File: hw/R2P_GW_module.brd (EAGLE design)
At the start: 40 x 40 mm, 32 parts, among them U1 STM32F103CX, U5 LD3985XX, X1 MICROMATCH-4

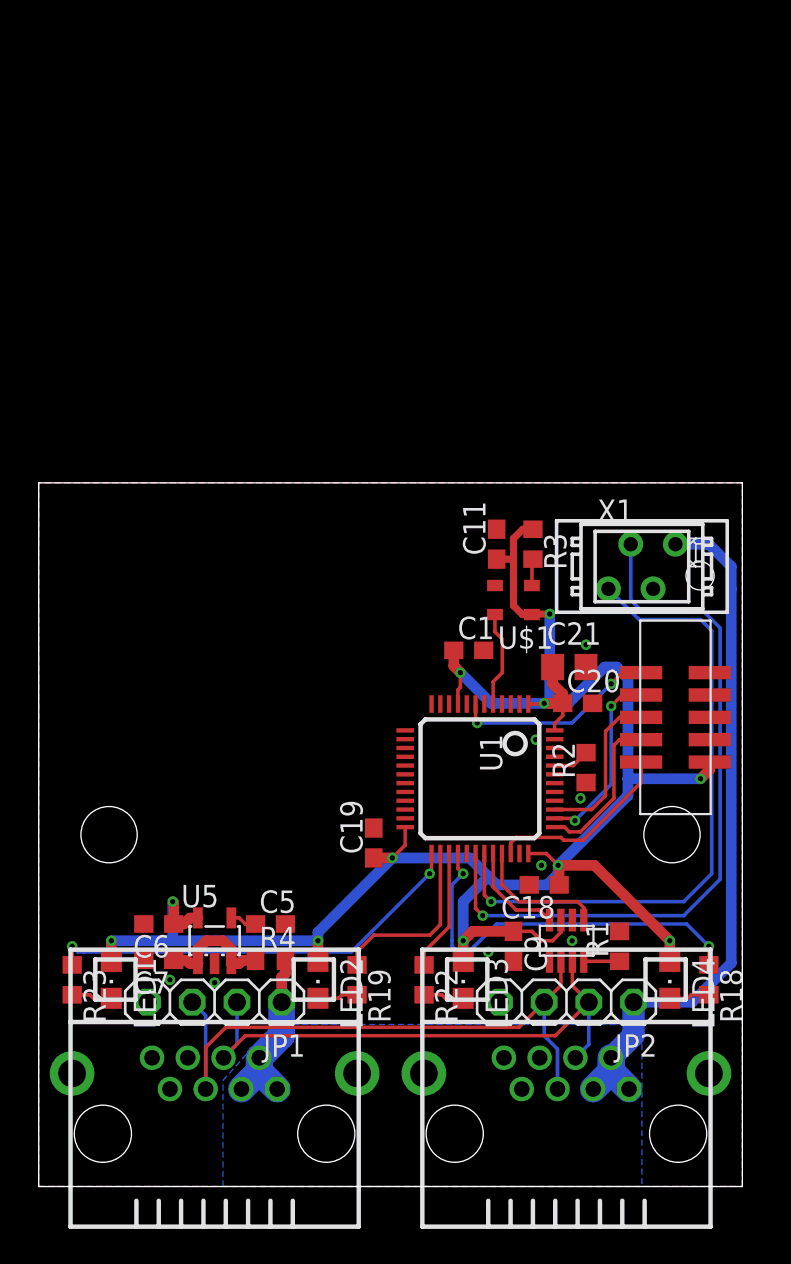
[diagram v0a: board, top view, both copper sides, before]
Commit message: First PCB version almost finished
Andrea Zoppi
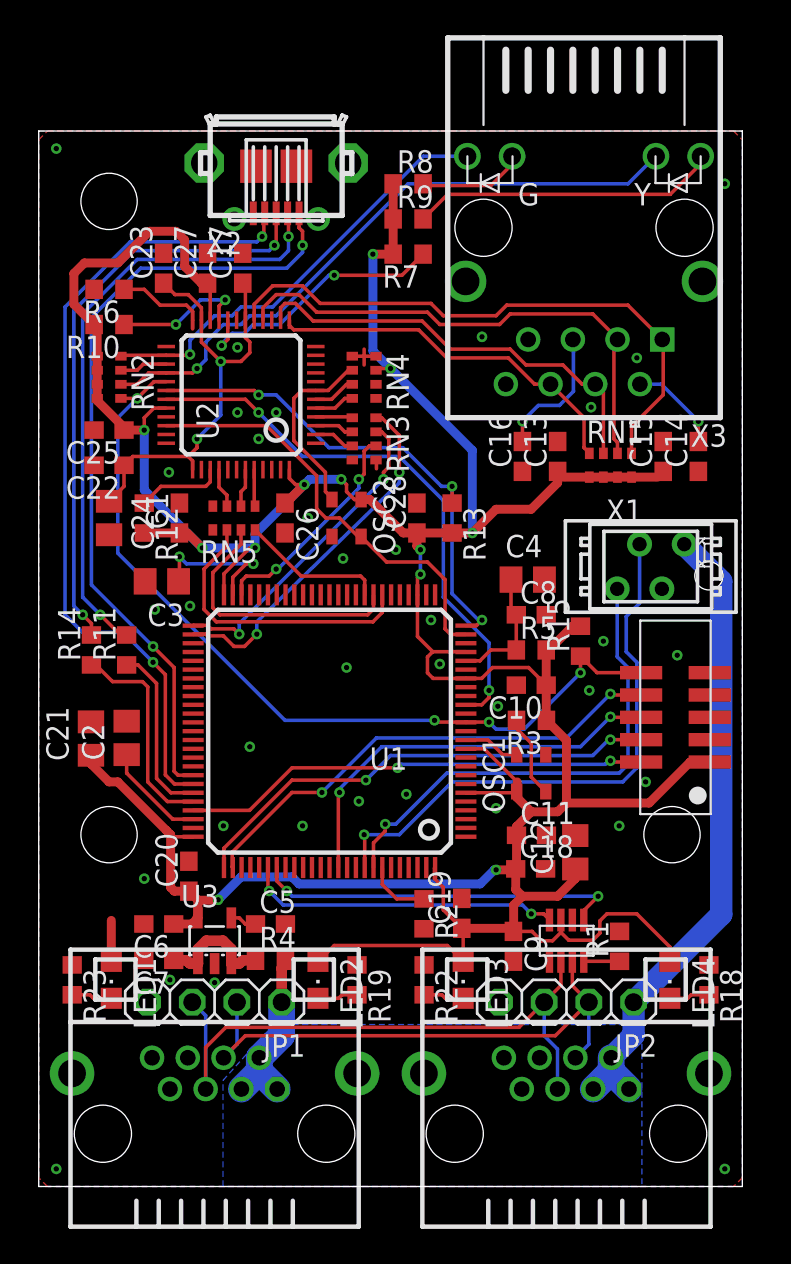
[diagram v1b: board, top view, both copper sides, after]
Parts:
- removed U$1: ASE, crystal:ASE
- added C10, C13, C14, C15, C16, C17, C22, C23, C25, C26, C27, C8: 100n, rcl:C0603
- added C12: 4u7, rcl:C0805
- added C2, C3: 2u2, rcl:C0805
- added C24: 10u, rcl:C0805
- added C28: 15p, rcl:C0603
- added C4: 1u, rcl:C0805
- added OSC1: ASE 8MHz, crystal:ASE
- added OSC2: ASE 50MHz, crystal:ASE
- added R10, R15, R7: 2k2, rcl:R0603
- added R11, R14: 22, rcl:R0603
- added R12: 100k, rcl:R0603
- added R13: 1k5, rcl:R0603
- added R5: 47, rcl:R0603
- added R6: 4k87, rcl:R0603
- added R8, R9: 220, rcl:R0603
- added RN1, RN3, RN5: 51, resistor-dil:CAT16
- added RN2, RN4: 2k2, resistor-dil:CAT16
- added U2: DP83848C, texas-instruments:LQFP48
- added X2: 47589-0001, molex:47589-0001
- added X3: (no value), bel:SI-60062-F
- C11: value 15pF -> 15p
- C21: value 4.7u -> 4u7
- R2: value 10k -> 100k
- U1: value STM32F103CX -> STM32F407VG; device st:LQFP48 -> st:LQFP100
- moved C21 27.5 mm to (2.97, 25.5), turned to 90 degrees
- moved C20 24.2 mm to (8.54, 17.6), turned to 90 degrees
- moved C1 18.1 mm to (8.00, 38.0), turned to 90 degrees
- moved C11 16.7 mm to (28.0, 20.0), turned to 0 degrees
- moved R2 12.4 mm to (21.9, 15.5), turned to 270 degrees
- moved R3 10.0 mm to (28.0, 26.5), turned to 180 degrees
- moved U1 8.57 mm to (17.0, 26.0), turned to 180 degrees
- moved C19 6.40 mm to (24.1, 15.5)
- moved C18 1.19 mm to (28.0, 18.1), turned to 0 degrees
- moved X1 0.50 mm to (34.8, 35.2)
- renumbered SOT1 to U4, U5 to U3
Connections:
- removed net AM_DRDY: U1.41
- removed net AM_INT1: U1.42
- removed net AM_INT2: U1.43
- removed net BOOT0: R2.2, U1.44
- removed net GPS_RESET: U1.14
- removed net GPS_RX: U1.13
- removed net GPS_STATUS: U1.11
- removed net GPS_TX: U1.12
- removed net GYRO_CS: U1.18
- removed net GYRO_INT1: U1.21
- removed net GYRO_INT2: U1.19
- removed net MISO: U1.16
- removed net MOSI: U1.17
- removed net NRST: U$4.P$10, U1.7
- removed net OSC_IN: U$1.3, U1.5
- removed net OSC_OUT: U1.6
- removed net SCK: U1.15
- removed net SCL: U1.45
- removed net SDA: U1.46
- new net !ETH_PWRDN: OSC2.1, RN4.6, U2.7
- new net !RESET: R15.1, RN2.1, U$4.10, U1.14, U2.29
- new net ETH_RMII_CRS_DV: RN5.2, U1.32
- new net ETH_RMII_MDC: U1.16, U2.31
- new net ETH_RMII_MDIO: R13.1, U1.25, U2.30
- new net ETH_RMII_REF_CLK: OSC2.3, U1.24, U2.34
- new net ETH_RMII_RXD0: RN5.3, U1.33
- new net ETH_RMII_RXD1: RN5.4, U1.34
- new net ETH_RMII_TXD0: RN3.3, U1.51
- new net ETH_RMII_TXD1: RN3.4, U1.52
- new net ETH_RMII_TXEN: RN3.2, U1.48
- new net MCU_CLK: OSC1.3, U1.12
- new net N$10: RN1.3, U2.14, X3.4
- new net N$11: RN1.4, U2.13, X3.6
- new net N$12: R9.2, X3.YA
- new net N$13: C14.2, X3.2
- new net N$14: C17.1, C22.1, C23.1, C24.1, U2.18, U2.23, U2.37
- new net N$16: C16.2, X3.5
- new net N$17: R8.2, X3.GA
- new net N$19: RN2.3, U2.27
- new net N$21: RN3.7, U2.2
- new net N$23: RN2.2, U2.28, X3.YK
- new net N$24: RN2.4, U2.26, X3.GK
- new net N$25: RN3.6, U2.3
- new net N$26: R2.1, U1.94
- new net N$27: R7.1, U2.20
- new net N$28: R10.1, U2.21
- new net N$29: RN3.5, U2.4
- new net N$30: RN4.8, U2.5
- new net N$31: RN4.7, U2.6
- new net N$32: R14.2, X2.3
- new net N$34: RN5.6, U2.43
- new net N$38: R12.1, U2.39
- new net N$40: RN5.5, U2.44
- new net N$41: RN5.7, U2.40
- new net N$6: R6.1, U2.24
- new net N$7: R11.2, X2.2
- new net N$8: RN1.1, U2.17, X3.1
- new net N$9: RN1.2, U2.16, X3.3
- new net USB_DM: R11.1, U1.70
- new net USB_DP: R14.1, U1.71
- new net USB_ID: U1.69, X2.4
- new net USB_VBUS: U1.68, X2.1
- new net VCAP_1: C3.1, U1.49
- new net VCAP_2: C2.1, U1.73
- net +3V3: now also C10.1, C12.1, C13.1, C15.1, C25.1, C26.1, C27.1, C28.1, OSC1.4, OSC2.4, R10.2, R12.2, R13.2, R15.2, R5.2, R7.2, R8.1, R9.1, RN1.5, RN1.6, RN1.7, RN1.8, RN2.5, RN2.6, RN2.7, RN2.8, RN4.3, U$4.1, U1.100, U1.11, U1.19, U1.22, U1.28, U1.50, U1.6, U1.75, U2.22, U2.32, U2.48; no longer U$1.4, U$4.P$1, U1.1, U1.24, U1.36, U1.48, U1.9
- net CAN_RX: now also U1.81; no longer U1.32
- net CAN_TX: now also U1.82; no longer U1.33
- net GND: now also C10.2, C12.2, C13.2, C14.1, C15.2, C16.1, C17.2, C2.2, C22.2, C23.2, C24.2, C25.2, C26.2, C27.2, C28.2, C3.2, C4.2, C8.2, OSC1.2, OSC2.2, R2.2, R6.2, RN3.1, RN3.8, RN4.1, RN4.2, RN4.4, RN4.5, RN5.1, RN5.8, U$4.3, U$4.5, U$4.9, U1.10, U1.20, U1.27, U1.74, U1.99, U2.15, U2.19, U2.35, U2.36, U2.47, X2.5, X2.SHLD1, X2.SHLD2, X2.SHLD3, X2.SHLD4, X3.8, X3.SHLD1, X3.SHLD2; no longer R2.1, U$1.2, U$4.P$3, U$4.P$9, U1.23, U1.35, U1.47, U1.8
- net JTCK: now also U$4.4, U1.76; no longer U$4.P$4, U1.37
- net JTDI: now also U$4.8, U1.77; no longer U$4.P$8, U1.38
- net JTDO: now also U$4.6, U1.89; no longer U$4.P$6, U1.39
- net JTMS: now also U$4.2, U1.72; no longer U$4.P$2, U1.34
- net LED1: no longer U1.25
- net LED2: no longer U1.26
- net LED3: no longer U1.27
- net LED4: no longer U1.28
- net N$1: now also C4.1, C8.1, R5.1, U1.21; no longer U$4.P$5
- net N$3: now also OSC1.1; no longer U$1.1
- net UART_RX: now also U1.93; no longer U1.31
- net UART_TX: now also U1.92; no longer U1.30
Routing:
- net +3V3: track 116.2 -> 229.6 mm, vias 11 -> 12
- net !RESET: track 0.00 -> 48.8 mm, vias 0 -> 4
- net USB_ID: track 0.00 -> 46.3 mm, vias 0 -> 2
- net USB_VBUS: track 0.00 -> 44.8 mm, vias 0 -> 2
- net N$23: track 0.00 -> 36.4 mm, vias 0 -> 1
- net N$7: track 0.00 -> 34.8 mm, vias 0 -> 2
- net N$32: track 0.00 -> 33.7 mm, vias 0 -> 2
- net N$8: track 0.00 -> 33.5 mm
- net ETH_RMII_MDC: track 0.00 -> 31.9 mm, vias 0 -> 2
- net N$9: track 0.00 -> 29.4 mm
- net ETH_RMII_MDIO: track 0.00 -> 28.9 mm, vias 0 -> 3
- net N$14: track 0.00 -> 25.5 mm, vias 0 -> 2
- net N$24: track 0.00 -> 24.9 mm, vias 0 -> 1
- net N$10: track 0.00 -> 24.7 mm
- net ETH_RMII_REF_CLK: track 0.00 -> 24.7 mm
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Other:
- board size 40 x 40 mm -> 40 x 60 mm
